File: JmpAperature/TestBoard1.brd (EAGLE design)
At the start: 160 x 100 mm, 4 parts

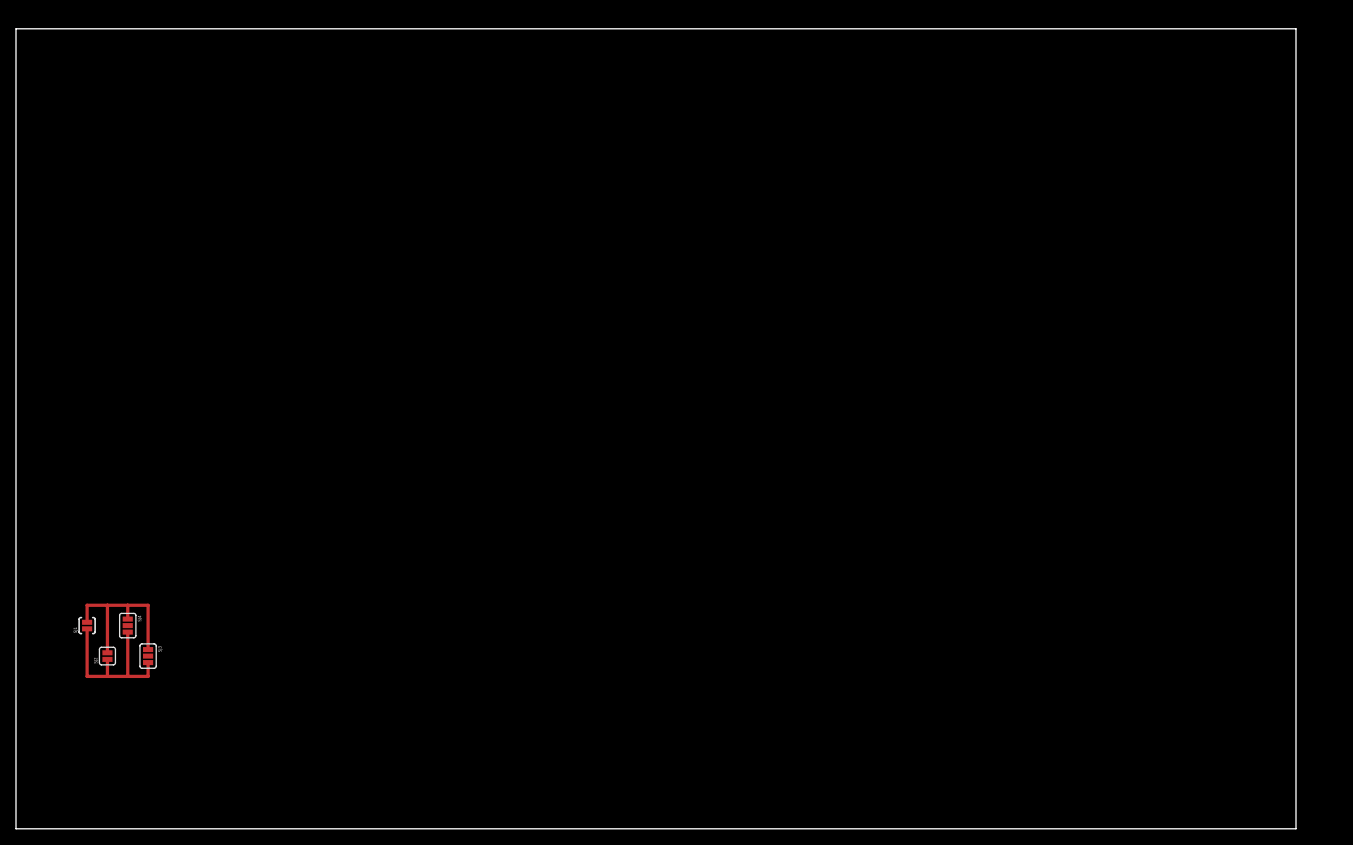
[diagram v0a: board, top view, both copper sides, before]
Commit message: updated
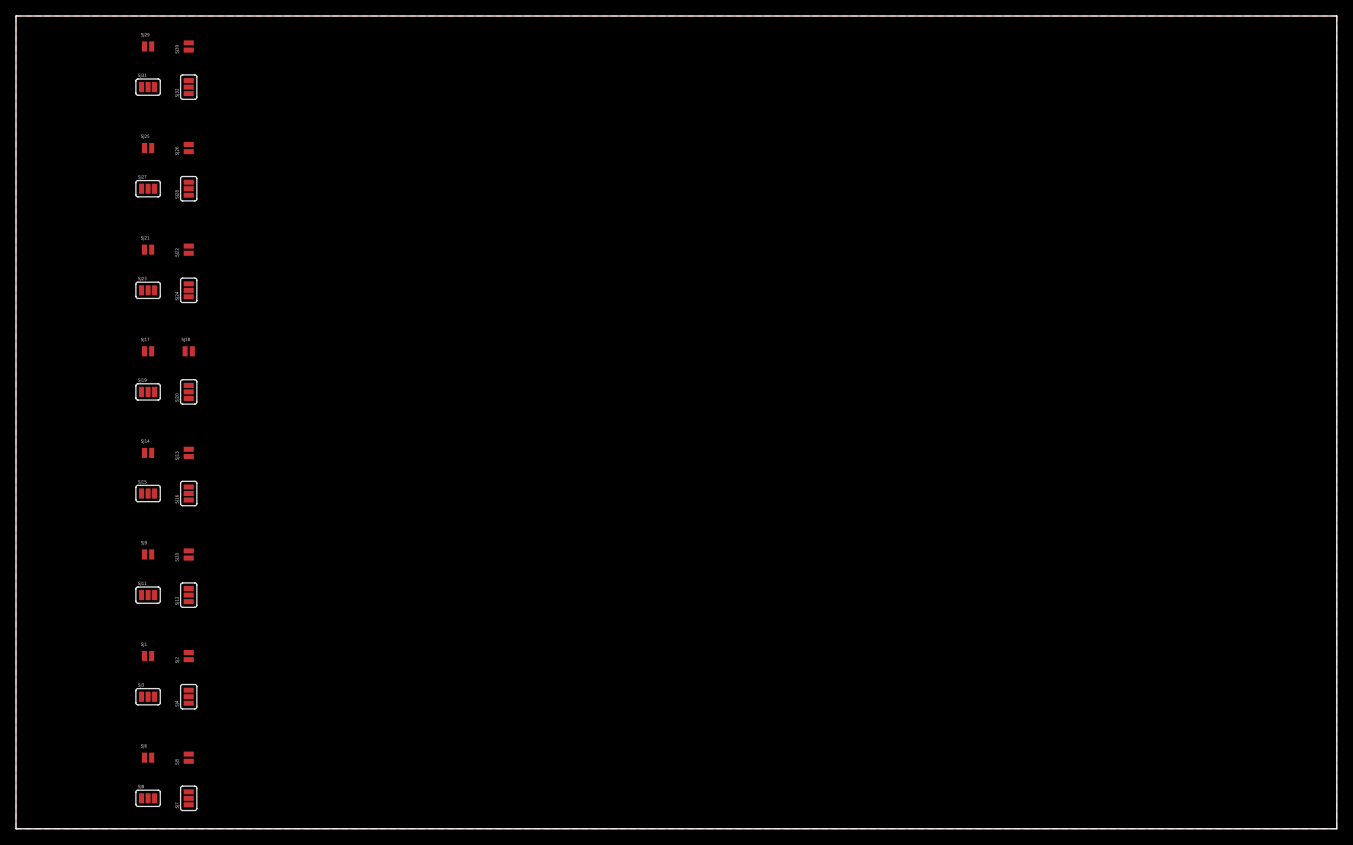
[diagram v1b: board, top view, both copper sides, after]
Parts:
- added SJ10, SJ13, SJ14, SJ17, SJ18, SJ21, SJ22, SJ25, SJ26, SJ29, SJ30, SJ5, SJ6, SJ9: JUMPER-PAD-2-NO, TestAperatures:PAD-JUMPER-2-NO_NO_SILK
- added SJ11, SJ12, SJ15, SJ16, SJ19, SJ20, SJ23, SJ24, SJ27, SJ28, SJ31, SJ32, SJ7, SJ8: JUMPER-PAD-3-NOYES_SILK, TestAperatures:PAD-JUMPER-3-NO_YES_SILK
- SJ1: value JUMPER-PAD-2-NC_BY_PASTE -> JUMPER-PAD-2-NO; device TestAperatures:PAD-JUMPER-2-NC_BY_PASTE_YES_SILK -> TestAperatures:PAD-JUMPER-2-NO_NO_SILK
- SJ2: value JUMPER-PAD-2-NC_BY_PASTEFULL-BOX-SILK -> JUMPER-PAD-2-NO; device TestAperatures:PAD-JUMPER-2-NC_BY_PASTE_YES_SILK_FULL_BOX -> TestAperatures:PAD-JUMPER-2-NO_NO_SILK
- SJ3: value JUMPER-PAD-3-2OF3_NC_BY_PASTE -> JUMPER-PAD-3-NOYES_SILK; device TestAperatures:PAD-JUMPER-3-2OF3_NC_BY_PASTE_YES_SILK_FULL_BOX -> TestAperatures:PAD-JUMPER-3-NO_YES_SILK
- SJ4: value JUMPER-PAD-3-NC_BY_PASTE -> JUMPER-PAD-3-NOYES_SILK; device TestAperatures:PAD-JUMPER-3-NC_BY_PASTE_YES_SILK_FULL_BOX -> TestAperatures:PAD-JUMPER-3-NO_YES_SILK
- moved SJ4 11.7 mm to (21.6, 16.5), turned to 90 degrees
- moved SJ2 10.2 mm to (21.6, 21.6)
- moved SJ1 8.52 mm to (16.5, 21.6), turned to 0 degrees
- moved SJ3 5.08 mm to (16.5, 16.5), turned to 0 degrees
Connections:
- removed net GND: SJ1.1, SJ2.1, SJ3.3, SJ4.3
- removed net PWR: SJ1.2, SJ2.2, SJ3.1, SJ4.1
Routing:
- net GND: track 23.0 -> 0.00 mm
- net PWR: track 22.9 -> 0.00 mm
- added copper zone on layer 1, net GND
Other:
- board size 160 x 100 mm -> 165.1 x 101.6 mm
- board text added: "10%"
- board text added: "20%"
- board text added: "30%"
- board text added: "40%"
- board text added: "50%"
- board text added: "60%"
- board text added: "70%"
- board text added: "Control"
